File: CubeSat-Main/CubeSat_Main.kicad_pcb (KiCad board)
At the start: 2 copper layers, 92 x 92 mm, 25 parts, among them J1 Conn_01x03_Pin, J2 Conn_01x08_Socket, U1 STM32F411CEU6 - BlackPill, U2 LORA E220-900T22D, U3 BNO055, U4 LM35-LP, U5 GPS_NEO6M

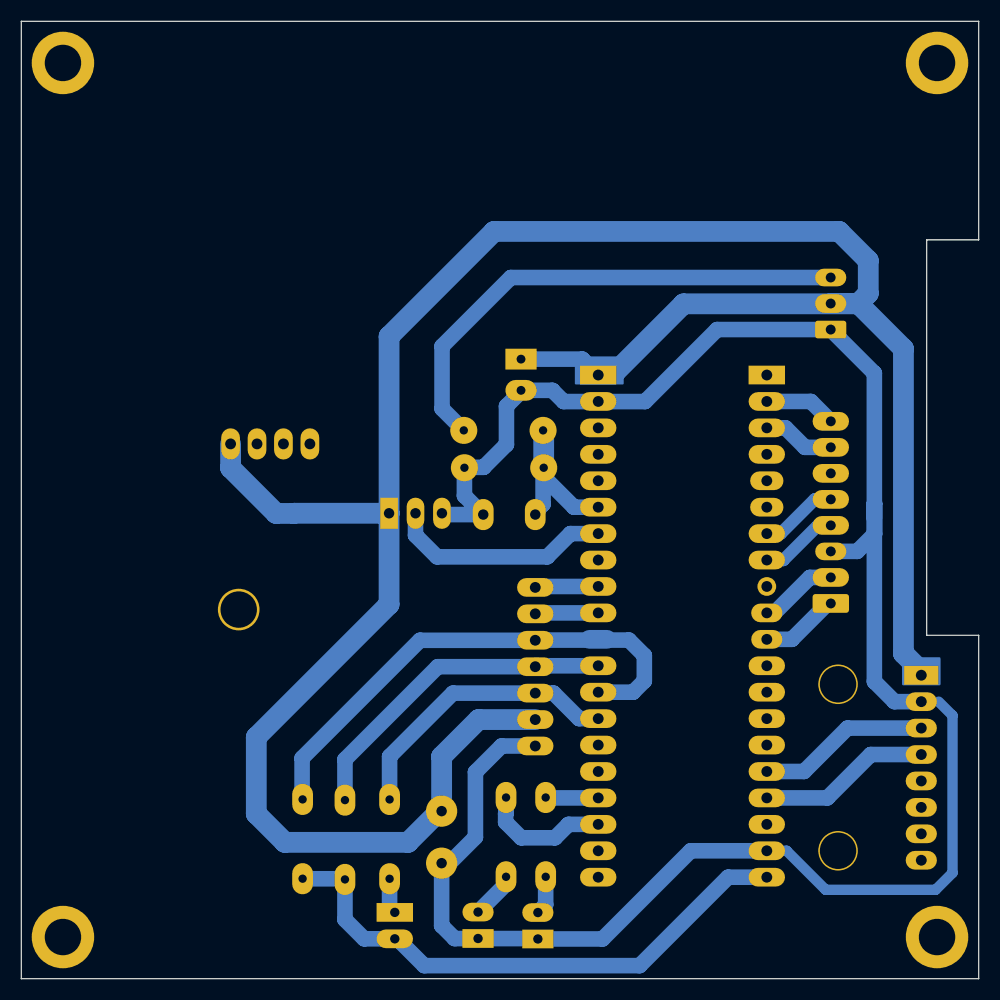
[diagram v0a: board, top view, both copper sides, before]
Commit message: minor changes in the design
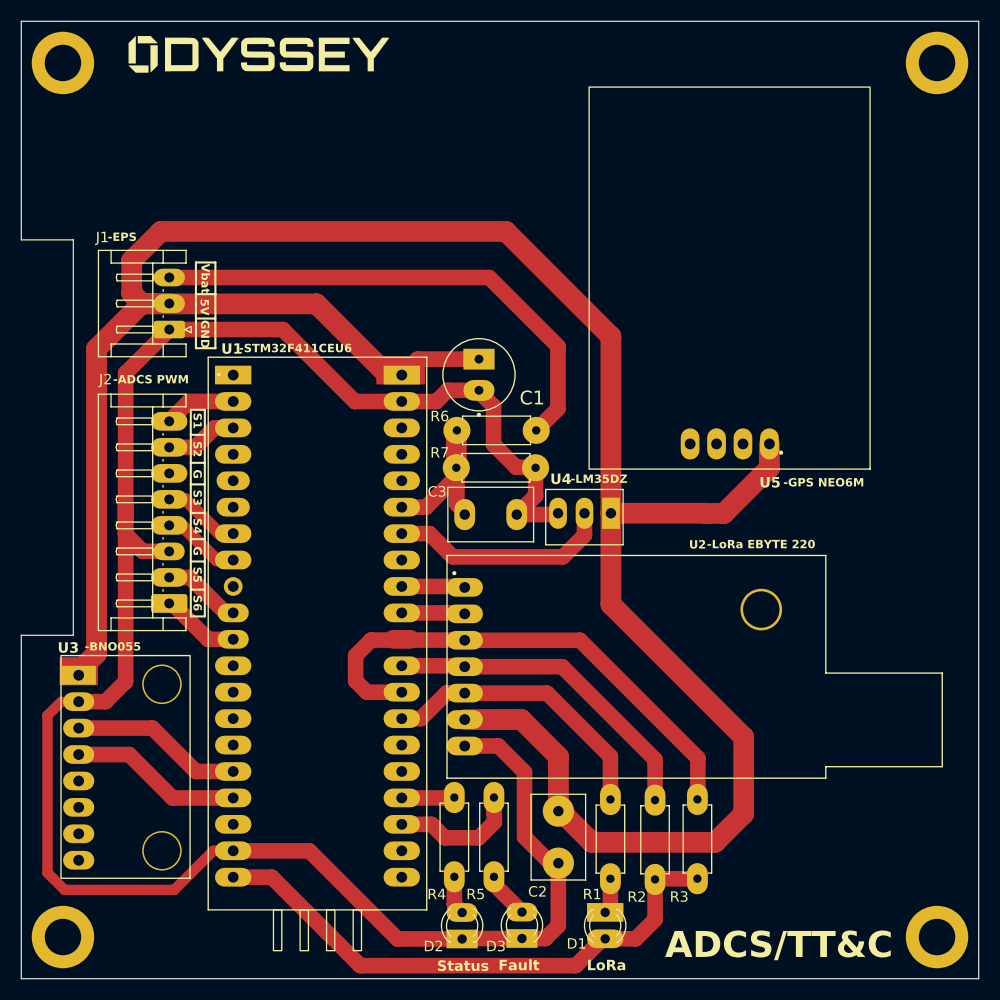
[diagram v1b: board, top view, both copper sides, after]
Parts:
- C1, C2, C3, D1, D2, D3, G***, J1, J2, R1, R2, R3, R4, R5, R6, R7, REF** (x4), U1, U2, U3, U4, U5: moved to F.Cu
- moved REF** 84.0 mm to (88.0, -4.00), turned to 0 degrees
- moved REF** 84.0 mm to (4.00, -4.00), turned to 0 degrees
- moved REF** 84.0 mm to (88.0, -88.0), turned to 0 degrees
- moved REF** 84.0 mm to (4.00, -88.0), turned to 0 degrees
- moved U3 72.0 mm to (10.0, -20.3), turned to 180 degrees
- moved J2 63.6 mm to (14.2, -36.1)
- moved J1 63.6 mm to (14.2, -62.4)
- moved G*** 46.2 mm to (22.9, -88.8), turned to 0 degrees
- moved U5 43.9 mm to (68.0, -66.9), turned to 180 degrees
- moved R3 37.9 mm to (65.0, -17.2)
- moved U1 35.1 mm to (28.5, -33.5), turned to 0 degrees
- moved R2 29.8 mm to (60.9, -17.2)
- moved U2 26.2 mm to (59.1, -30.0)
- moved R1 21.2 mm to (56.6, -17.2)
- moved D1 20.2 mm to (56.1, -6.37)
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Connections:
- R4 pad 1: LED_RED -> LED_BLUE
- R5 pad 1: LED_BLUE -> LED_RED
- U1 pad 3: LED_BLUE -> LED_RED
- U1 pad 4: LED_RED -> LED_BLUE
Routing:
- net LED_RED: track 5.65 -> 12.4 mm
- net LED_BLUE: track 12.4 -> 5.65 mm
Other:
- outline, holes or cut-outs redrawn
